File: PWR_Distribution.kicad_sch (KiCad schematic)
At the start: 35 parts, among them IC3 LM74502HDDFR, IC4 AP64501QSP-13, J1 CarLVPowerConnector, J2 Display Breakout, Q1 PSMN8R5-40MSDX

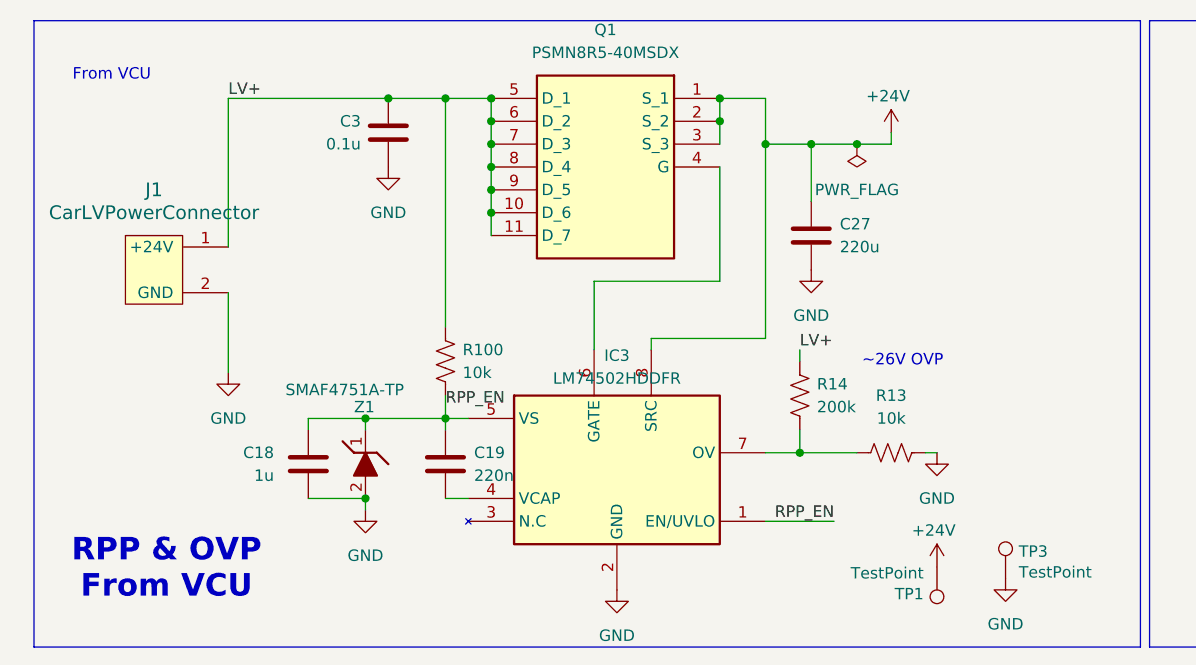
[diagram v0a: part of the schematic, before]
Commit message: frank
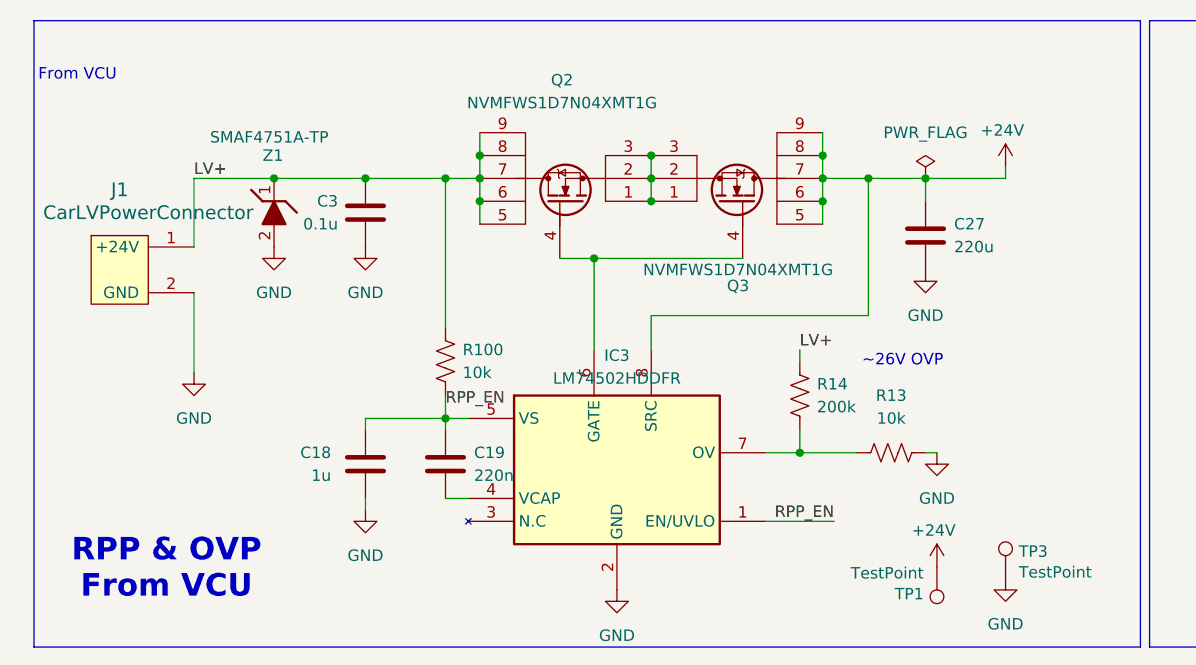
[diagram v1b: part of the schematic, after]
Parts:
- removed Q1: PSMN8R5-40MSDX, UTSVT_Power:PSMN8R5-40MSDX, symbol utsvt_power:PSMN8R5-40MSDX
- added Q2, Q3: NVMFWS1D7N04XMT1G, Controls_Pi:NVMFWS3D0P04M8LT1G, symbol NVMFWS1D7N04XMT1G:NVMFWS1D7N04XMT1G
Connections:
- net +24V: now also Q3.5, Q3.6, Q3.7, Q3.8, Q3.9
- net LV+: now also Z1.1 (K), Q2.5, Q2.6, Q2.7, Q2.8, Q2.9
- net RPP_EN: no longer Z1.1 (K)
- net at IC3.6 (GATE): now also Q2.4, Q3.4
- new net: Q2.1, Q2.2, Q2.3, Q3.1, Q3.2, Q3.3
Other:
- moved on the sheet: C18, C27, C3, J1, Z1
